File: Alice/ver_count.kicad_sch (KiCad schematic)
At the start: 315 parts, among them Q10 NOT_OC, Q100 NOT_OC, Q101 NOT_OC, Q102 NOT_OC, Q103 NOT_OC, Q104 NOT_OC, Q105 NOT_OC, Q106 NOT_OC, Q107 NOT_OC, Q108 NOT_OC, Q109 NOT_OC, Q11 NOT_OC, Q110 NOT_OC, Q111 NOT_OC, Q112 NOT_OC, Q113 NOT_OC, Q114 NOT_OC, Q115 NOT_OC, Q116 NOT_OC, Q117 NOT_OC, Q118 NOT_OC, Q119 NOT_OC, Q12 NOT_OC, Q120 NOT_OC, Q121 NOT_OC, Q122 NOT_OC, Q123 NOT_OC, Q124 NOT_OC, Q125 NOT_OC, Q126 NOT_OC, Q127 NOT_OC, Q128 NOT_OC, Q129 NOT_OC, Q13 NOT_OC, Q130 NOT_OC, Q131 NOT_OC, Q132 NOT_OC, Q133 NOT_OC, Q134 NOT_OC, Q135 NOT_OC, Q136 NOT_OC, Q137 NOT_OC, Q138 NOT_OC, Q139 NOT_OC, Q14 NOT_OC, Q140 NOT_OC, Q141 NOT_OC, Q142 NOT_OC, Q143 NOT_OC, Q144 NOT_OC, Q145 NOT_OC, Q146 NOT_OC, Q147 NOT_OC, Q148 NOT_OC, Q149 NOT_OC, Q15 NOT_OC, Q150 NOT_OC, Q151 NOT_OC, Q152 NOT_OC, Q153 NOT_OC, Q154 NOT_OC, Q155 NOT_OC, Q156 NOT_OC, Q157 NOT_OC, Q158 NOT_OC, Q16 NOT_OC, Q17 NOT_OC, Q18 NOT_OC, Q19 NOT_OC, Q20 NOT_OC, Q21 NOT_OC, Q22 NOT_OC, Q23 NOT_OC, Q24 NOT_OC, Q25 NOT_OC, Q26 NOT_OC, Q27 NOT_OC, Q270 NOT_OC, Q271 NOT_OC, Q272 NOT_OC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

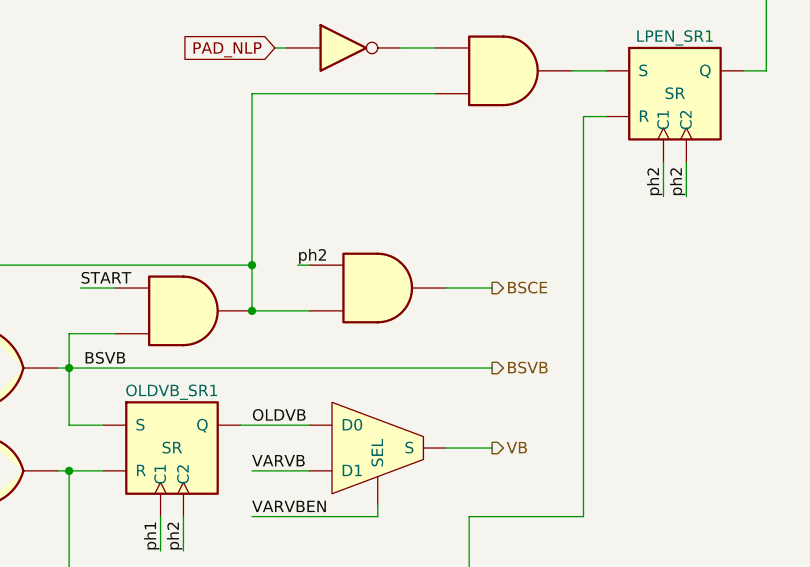
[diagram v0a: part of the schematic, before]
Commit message: Copper DMA done
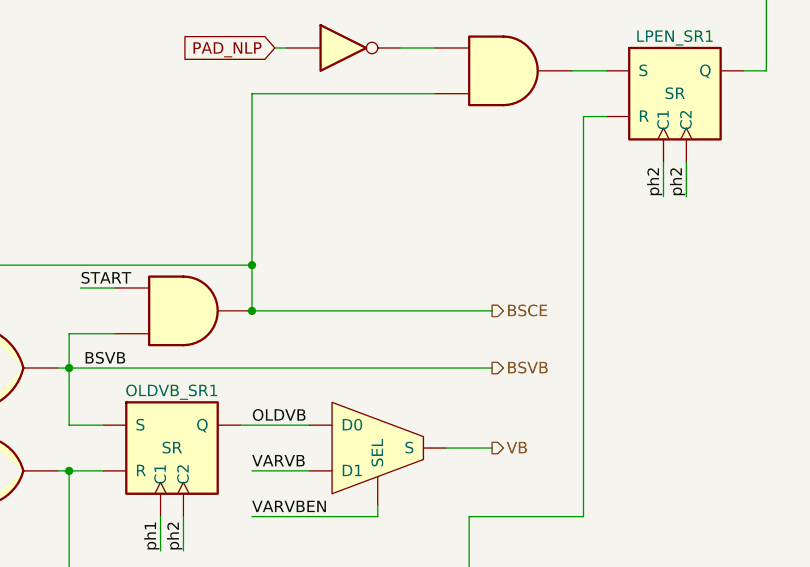
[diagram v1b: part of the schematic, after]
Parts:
- removed AND_39: AND2, symbol NMOS:AND2
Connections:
- net BSCE: now also AND_37.1, AND_40.3, VCT0.4 (M), VCT1.4 (M), VCT10.4 (M), VCT2.4 (M), VCT3.4 (M), VCT4.4 (M), VCT5.4 (M), VCT6.4 (M), VCT7.4 (M), VCT8.4 (M), VCT9.4 (M)
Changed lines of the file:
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@@
     (stroke (width 0) (type default) (color 0 0 0 0))
   )
-  (wire (pts (xy 359.41 87.63) (xy 360.68 87.63))
-    (stroke (width 0) (type default) (color 0 0 0 0))
-  )
   (wire (pts (xy 346.71 220.98) (xy 346.71 217.17))
     (stroke (width 0) (type default) (color 0 0 0 0))
@@
     (stroke (width 0) (type default) (color 0 0 0 0))
   )
-  (wire (pts (xy 375.92 90.17) (xy 381 90.17))
-    (stroke (width 0) (type default) (color 0 0 0 0))
-  )
   (wire (pts (xy 222.25 118.11) (xy 241.3 118.11))
     (stroke (width 0) (type default) (color 0 0 0 0))
@@
     (stroke (width 0) (type default) (color 0 0 0 0))
   )
-  (wire (pts (xy 360.68 92.71) (xy 354.33 92.71))
+  (wire (pts (xy 354.33 92.71) (xy 381 92.71))
     (stroke (width 0) (type default) (color 0 0 0 0))
   )
@@
     (effects (font (size 1.27 1.27)) (justify left bottom))
   )
-  (label "ph2" (at 359.41 87.63 0)
-    (effects (font (size 1.27 1.27)) (justify left bottom))
-  )
   (label "VSYTRUE" (at 358.14 292.1 0)
     (effects (font (size 1.27 1.27)) (justify left bottom))
@@
     (effects (font (size 1.27 1.27)) (justify right))
   )
-  (hierarchical_label "BSCE" (shape output) (at 381 90.17 0)
+  (hierarchical_label "BSCE" (shape output) (at 381 92.71 0)
     (effects (font (size 1.27 1.27)) (justify left))
   )
@@
     (pin "9")
   )
-  (symbol (lib_id "NMOS:AND2") (at 368.3 90.17 0) (unit 1)
-    (in_bom yes) (on_board yes) (fields_autoplaced)
-    (property "Reference" "AND_39" (id 0) (at 368.3 90.17 0)
-      (effects (font (size 1.27 1.27)) hide)
-    )
-    (property "Value" "AND2" (id 1) (at 368.3 95.25 0)
-      (effects (font (size 1.27 1.27)) hide)
-    )
-    (property "Footprint" "" (id 2) (at 368.3 90.17 0)
-      (effects (font (size 1.27 1.27)) hide)
-    )
-    (property "Datasheet" "" (id 3) (at 368.3 90.17 0)
-      (effects (font (size 1.27 1.27)) hide)
-    )
-    (pin "1")
-    (pin "2")
-    (pin "3")
-  )
   (symbol (lib_id "NMOS:NOT_OC") (at 116.84 114.3 0) (unit 1)
